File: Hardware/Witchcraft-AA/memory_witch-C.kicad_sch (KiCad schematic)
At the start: 1 part, among them U1 Z1 extreme

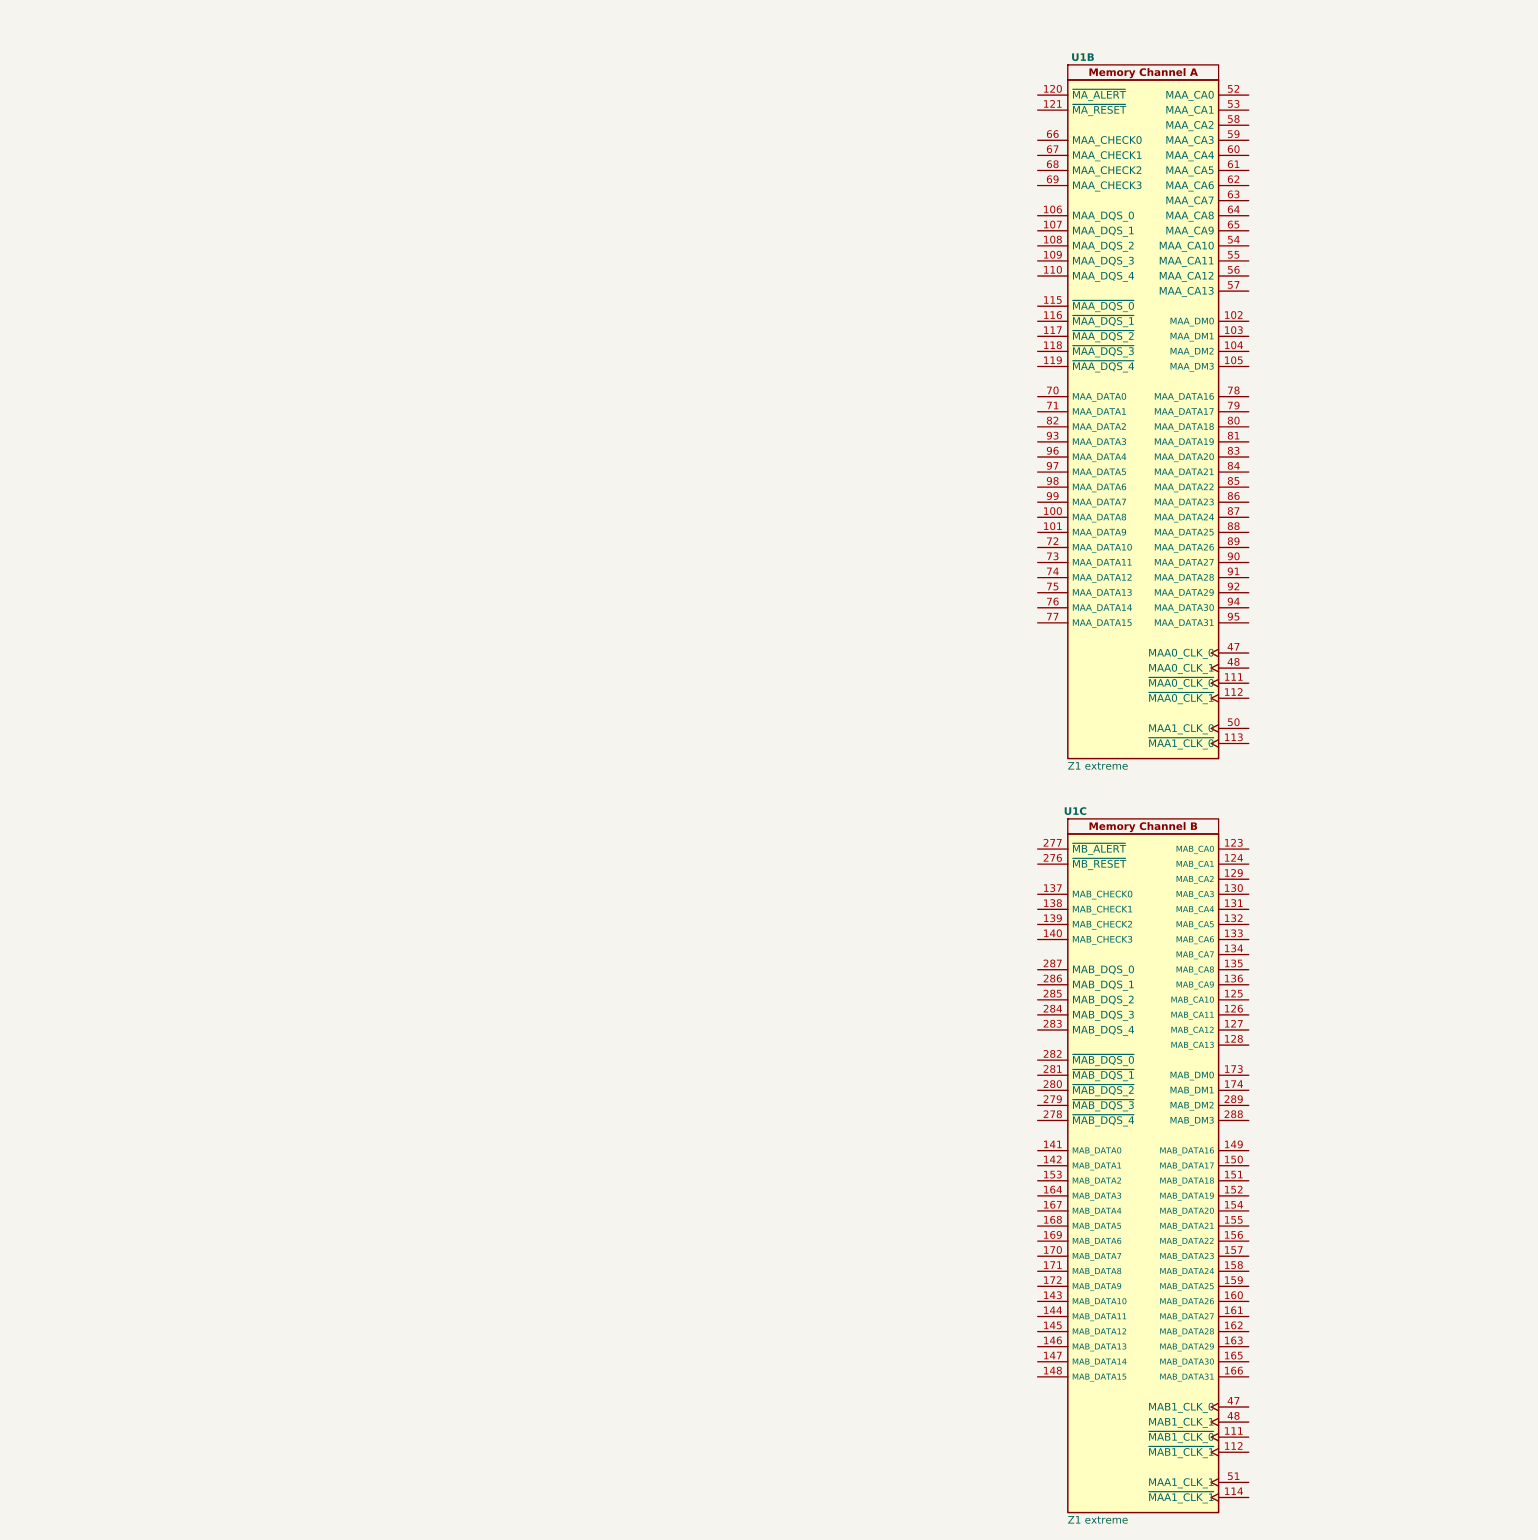
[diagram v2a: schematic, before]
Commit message: Some chances to start/rectangle-buttons in mech, and startedmaking the M.2 ports.
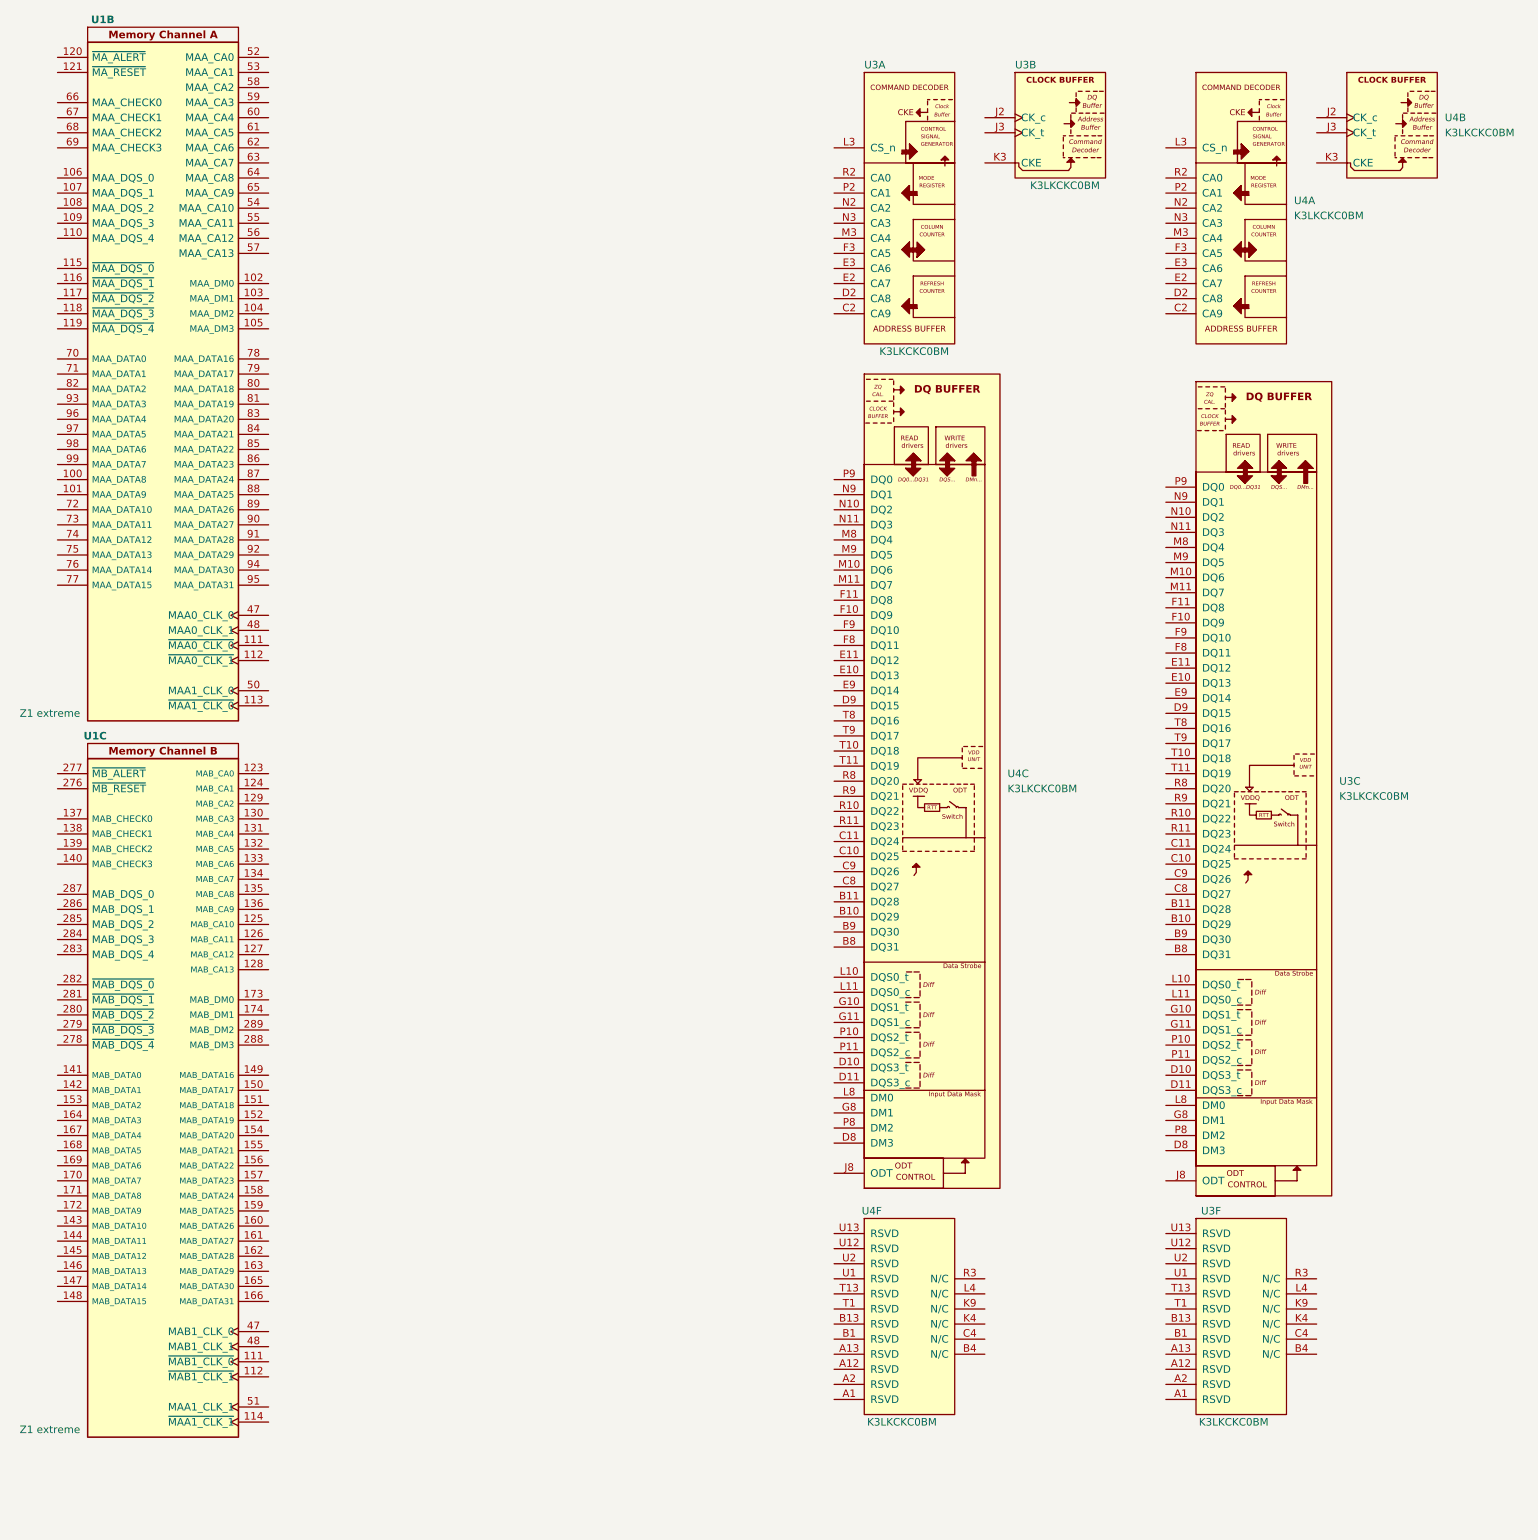
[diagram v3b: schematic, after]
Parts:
- added U3, U4: K3LKCKC0BM, LRJ:SAMSUNG_FBGA-315_12x14mm_Layout23x23_P0.5mmP0.65mm, symbol LRJ-parts:K3LKCKC0BM-MFCP
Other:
- moved on the sheet: U1B, U1C
